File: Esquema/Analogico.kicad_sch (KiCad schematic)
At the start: 39 parts, among them J1 Conex_bat, J2 Panel Solar, J3 Galga_1, J4 Galga_2, J5 Conn_01x02, P1 USB_C_Plug_USB2.0, U1 REF3020AIDBZT, U2 TMUX154EDGS, U3 TP4057, U4 INA826AIDR, U5 INA826AIDR, U6 XL006, U7 TLV75733PDBV, U8 TLV75733PDBV, U9 NUCLEO-F429ZI

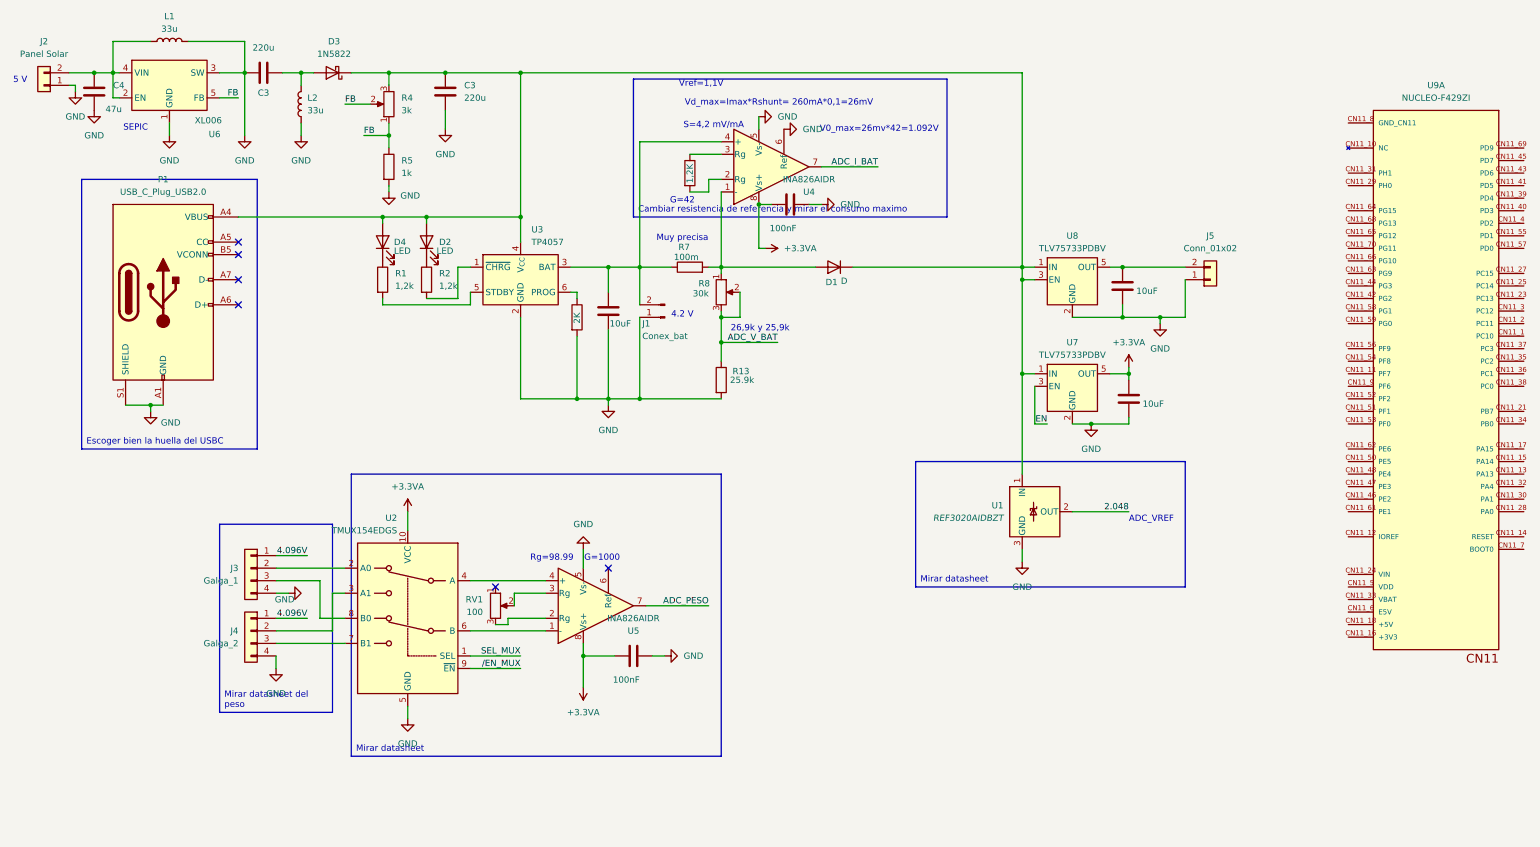
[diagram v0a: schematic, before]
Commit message: Huellas y componentes ya asignados
Signed-off-by: ricardo.socorro <ricardo.socorro@alumnos.upm.es>
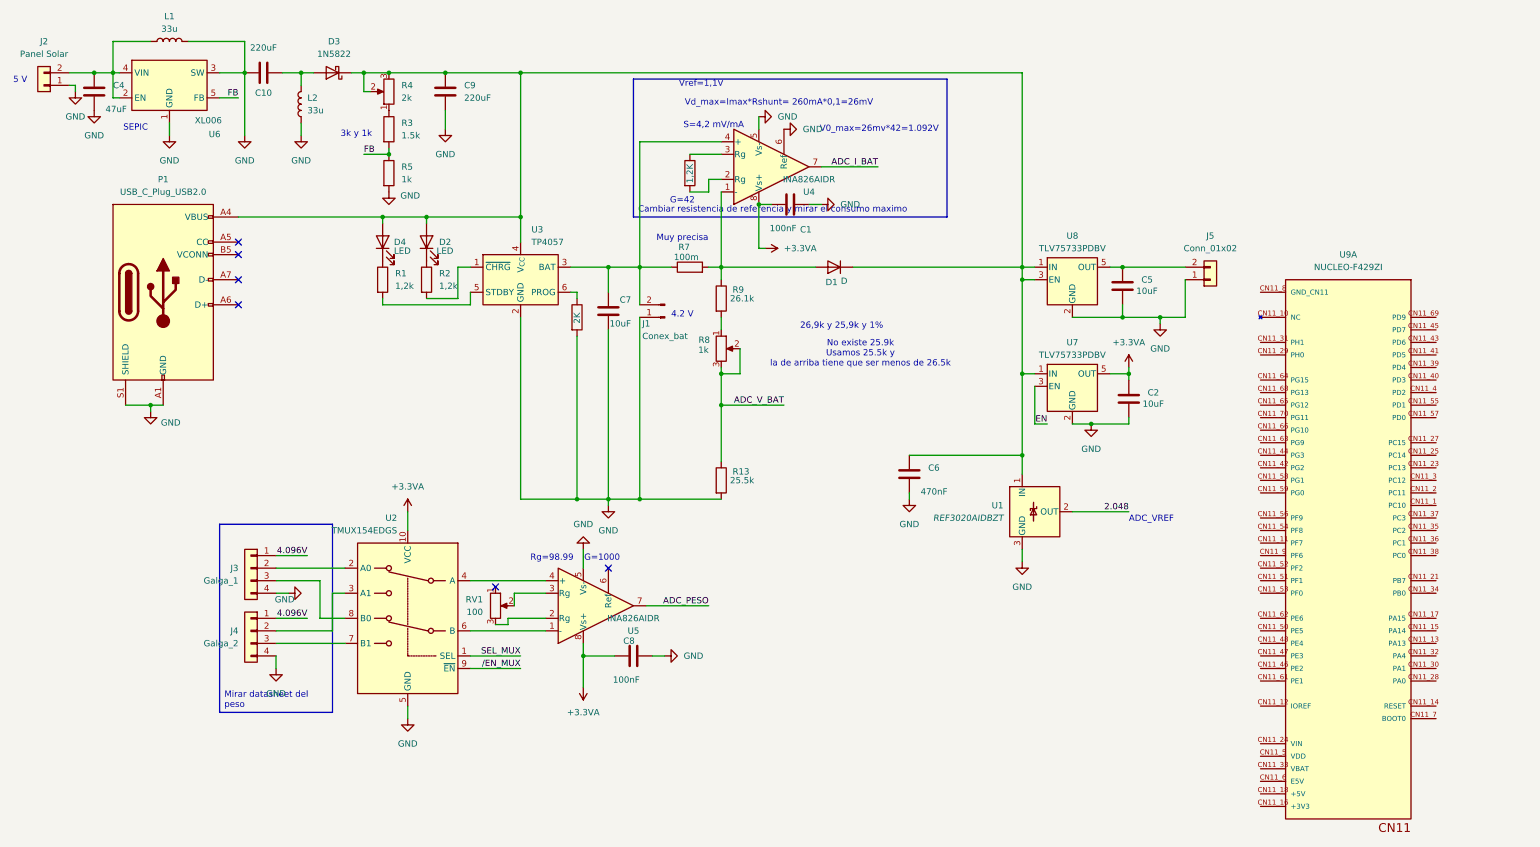
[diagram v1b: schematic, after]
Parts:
- added C6: 470nF, Capacitor_SMD:C_0805_2012Metric, symbol Device:C
- added R3: 1.5k, Resistor_SMD:R_0805_2012Metric, symbol Device:R
- added R9: 26.1k, Resistor_SMD:R_0805_2012Metric, symbol Device:R
- C10: renamed from C3; value 220u -> 220uF; footprint (none) -> Capacitor_SMD:C_1206_3216Metric; JLC (none) -> C412252
- C4: value 47u -> 47uF
- C9: renamed from C3; value 220u -> 220uF; JLC (none) -> C412252
- D2, D4: footprint (none) -> LED_THT:LED_D3.0mm; JLC (none) -> C85161
- J1: footprint (none) -> Connector_JST:JST_PH_S2B-PH-K_1x02_P2.00mm_Horizontal
- J2, J3, J4, J5: footprint (none) -> TerminalBlock_4Ucon:TerminalBlock_4Ucon_1x02_P3.50mm_Horizontal; JLC (none) -> C695629
- P1: footprint (none) -> Connector_USB:USB_C_Plug_ShenzhenJingTuoJin_918-118A2021Y40002_Vertical
- R1, R2: footprint (none) -> Resistor_SMD:R_0805_2012Metric; JLC (none) -> C114526
- R13: value 25.9k -> 25.5k
- R4: value 3k -> 2k; footprint (none) -> Potentiometer_THT:Potentiometer_Bourns_3266Y_Vertical; JLC (none) -> C48997938
- R5: footprint (none) -> Resistor_SMD:R_0805_2012Metric
- R8: value 30k -> 1k; footprint (none) -> Potentiometer_THT:Potentiometer_Bourns_3266Y_Vertical; JLC (none) -> C48997938
- RV1: footprint (none) -> Potentiometer_THT:Potentiometer_Bourns_3266Y_Vertical; JLC (none) -> C48997939
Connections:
- net FB: now also R3.2; no longer R4.1, R4.2
- net GND: now also C6.2
- net at D1.2 (A), R7.2, U4.1 (-): now also R9.1; no longer R8.1
- net at C9.1, D1.1 (K), D2.2 (A)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: now also R4.2, C6.1
- new net: R3.1, R4.1
- new net: R8.1, R9.2
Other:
- note added: "26,9k y 25,9k y 1%"
- note added: "3k y 1k"
- note added: "No existe 25.9k Usamos 25.5k y la de arriba tiene que ser menos de 26.5k"
- note removed: "26,9k y 25,9k"
- moved on the sheet: R13, R4, R5, R8, U9A

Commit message: PCB 1.0
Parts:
- removed J5: Conn_01x02, TerminalBlock_4Ucon:TerminalBlock_4Ucon_1x02_P3.50mm_Horizontal, symbol Connector_Generic:Conn_01x02
- removed U2: TMUX154EDGS, Package_SO:VSSOP-10_3x3mm_P0.5mm, symbol Analog_Switch:TMUX154EDGS
- removed U9: NUCLEO-F429ZI, stm32f429zi_symbol_footprint:MODULE_NUCLEO-F429ZI, symbol NUCLEO-F429ZI:NUCLEO-F429ZI
- added C3: 100nF, Capacitor_SMD:C_0805_2012Metric, symbol Device:C
- added RV2: 100, Potentiometer_THT:Potentiometer_Bourns_3266Y_Vertical, symbol Device:R_Potentiometer
- added U10: NUCLEO-F429ZI, mis_footprints:MODULE_NUCLEO-F429ZI_FEMALE, symbol mis_componentes:NUCLEO-F429ZI_FEMALE
- added U2: INA826AIDR, Package_SO:SOIC-8_3.9x4.9mm_P1.27mm, symbol Amplifier_Instrumentation:INA849D
- added U9: NUCLEO-F429ZI, NUCLEO-F429ZI:MODULE_NUCLEO-F429ZI, symbol mis_componentes:NUCLEO-F429ZI
- J3, J4: footprint TerminalBlock_4Ucon:TerminalBlock_4Ucon_1x02_P3.50mm_Horizontal -> TerminalBlock:TerminalBlock_MaiXu_MX126-5.0-04P_1x04_P5.00mm; JLC C695629 -> C192769
- P1: footprint Connector_USB:USB_C_Plug_ShenzhenJingTuoJin_918-118A2021Y40002_Vertical -> Connector_USB:USB_C_Receptacle_GCT_USB4125-xx-x-0190_6P_TopMnt_Horizontal
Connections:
- net 4.096V is gone; now on net 2.048: J3.1 (Pin_1), J4.1 (Pin_1)
- net +3.3VA: now also C3.1, U2.8 (Vs+)
- net 2.048: now also U10.CN10_1 (AVDD_CN10), U10.CN7_6 (AREF), U9.CN10_1 (AVDD_CN10)
- net ADC_I_BAT: now also U10.CN9_5 (A2/ADC123_IN13)
- net EN: now also U10.CN7_20 (D8/IO)
- net GND: now also C3.2, U10.CN10_17 (GND_CN10), U10.CN10_22 (GND_CN10), U10.CN10_27 (GND_CN10), U10.CN10_3 (AGND_CN10), U10.CN10_5 (GND_CN10), U10.CN7_8 (GND_CN7), U10.CN8_11 (GND_CN8), U10.CN8_13 (GND_CN8), U10.CN9_12 (GND_CN9), U10.CN9_23 (GND_CN9), U2.5 (Vs-), U9.CN10_17 (GND_CN10), U9.CN10_22 (GND_CN10), U9.CN10_27 (GND_CN10), U9.CN10_3 (AGND_CN10), U9.CN10_5 (GND_CN10)
- net at J4.2 (Pin_2): now also U2.4 (+)
- net at J4.3 (Pin_3): now also U2.1 (-)
- net at J3.2 (Pin_2): now also U5.4 (+)
- net at U5.1 (-): now also J3.3 (Pin_3)
- net +3.3V: now reaches C5.1, U8.5 (OUT)
- net +3.3V: now also U10.CN8_7 (+3V3_CN8)
- net ADC_PESO renamed ADC_PESO_1
- net ADC_PESO_1: now also U10.CN9_1 (A0/ADC123_IN3)
- new net: RV2.3, U2.2 (Rg)
- new net: RV2.2, U2.3 (Rg)
- new net ADC_PESO_2: U10.CN9_3 (A1/ADC123_IN10), U2.7
- no-connect marks 6 -> 120
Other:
- moved on the sheet: J3, J4
